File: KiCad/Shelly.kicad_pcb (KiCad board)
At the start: 2 copper layers, 16 x 30 mm, 15 parts, among them J1 Shelly 1, J2 Shelly 2, J3 Shelly i3, J4 USB-C, M1 D24V5F3-NoSHDN, U1 FT231XQ, U2 TLP3546

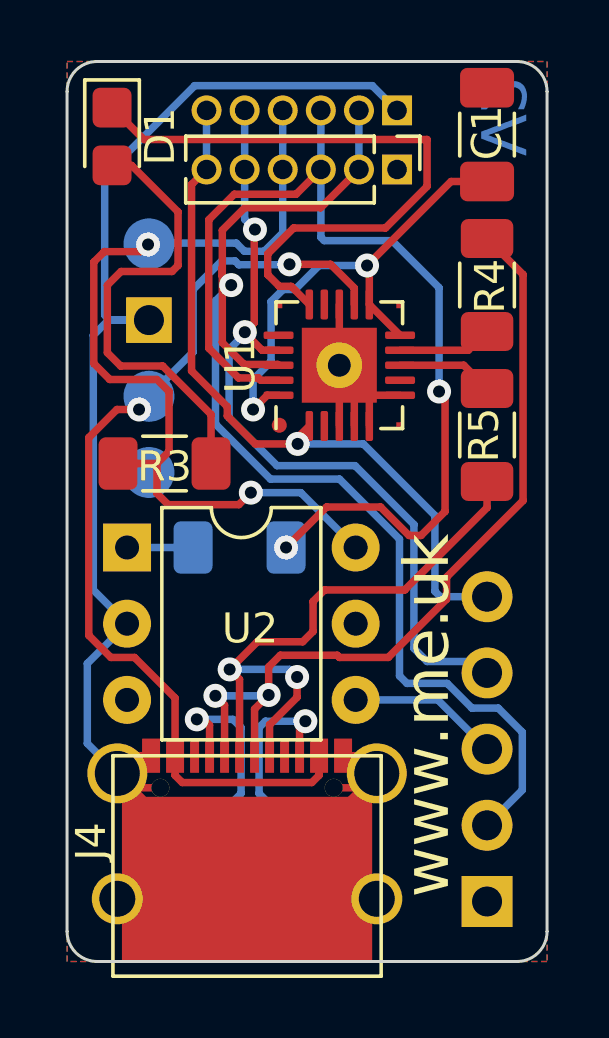
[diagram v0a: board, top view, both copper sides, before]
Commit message: FT231XQ
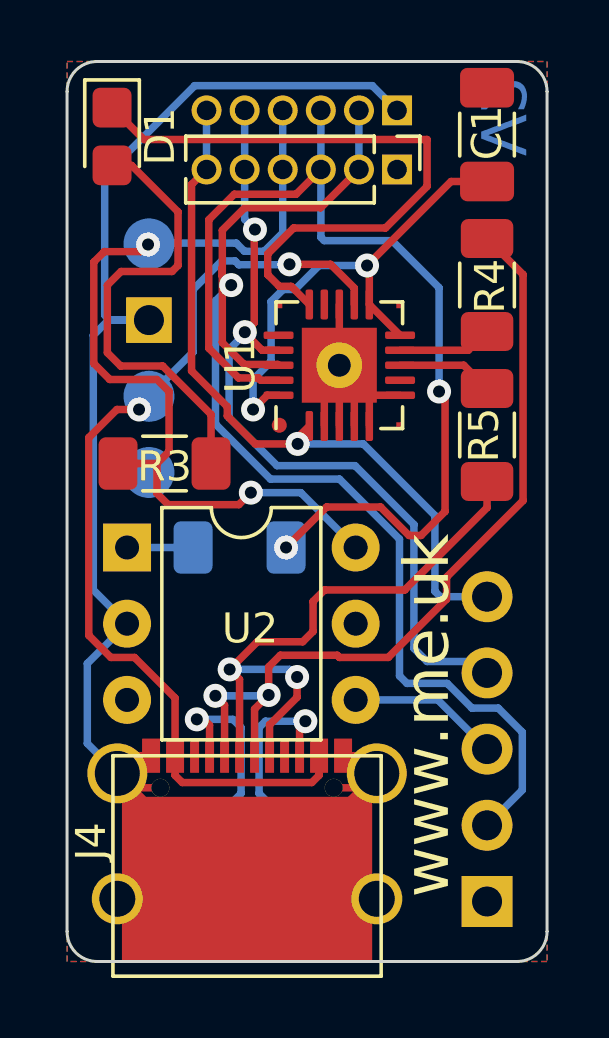
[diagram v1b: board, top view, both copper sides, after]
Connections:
- U1 pad 2: Net-(U1-Pad2) -> GND
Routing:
- net GND: track 67.5 -> 69.8 mm
